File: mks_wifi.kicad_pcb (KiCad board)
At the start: 2 copper layers, 22.4 x 21.6 mm, 4 parts, among them J1 Conn_01x08, J2 Conn_01x08, U1 ESP-12F

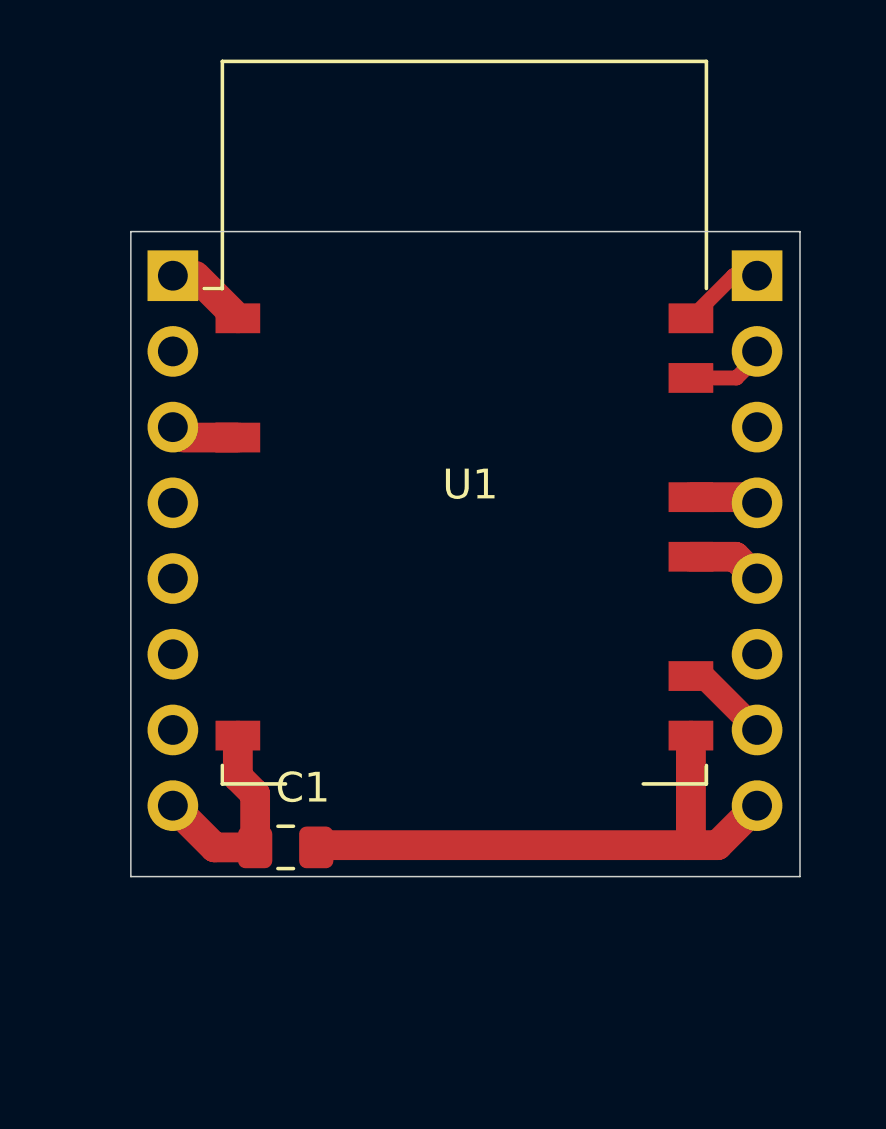
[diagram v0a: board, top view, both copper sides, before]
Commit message: v1, проверенный вариант
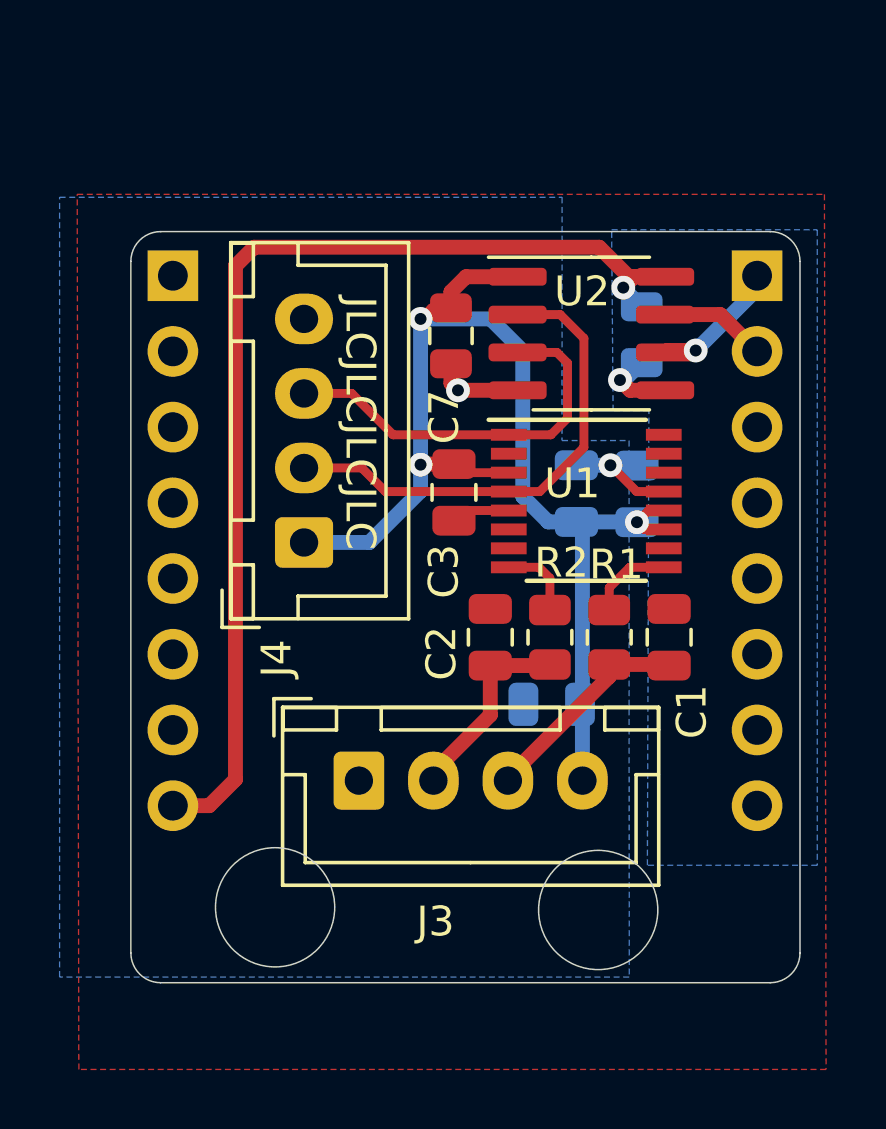
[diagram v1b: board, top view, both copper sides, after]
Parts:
- added C2: 47pF, Capacitor_SMD:C_0805_2012Metric, F.Cu at (174.6, 62.1)
- added C3: 0.1uF, Capacitor_SMD:C_0805_2012Metric, F.Cu at (173.4, 57.2)
- added C4: 4.7uF, Capacitor_SMD:C_0805_2012Metric, B.Cu at (177.5, 57.3)
- added C5: 0.1uF, Capacitor_SMD:C_0805_2012Metric, B.Cu at (179.5, 57.3)
- added C6: 0.01uF, Capacitor_SMD:C_0805_2012Metric, B.Cu at (176.7, 64.3)
- added C7: 1uF, Capacitor_SMD:C_0805_2012Metric, F.Cu at (173.3, 52.0)
- added C8: 1uF, Capacitor_SMD:C_0805_2012Metric, B.Cu at (179.7, 51.9)
- added J3: USB, Connector_JST:JST_XH_B4B-XH-A_1x04_P2.50mm_Vertical, F.Cu at (170.2, 66.9)
- added J4: UART, Connector_JST:JST_XH_B4B-XH-A_1x04_P2.50mm_Vertical, F.Cu at (168.4, 58.9)
- added R1: 27, Resistor_SMD:R_0805_2012Metric, F.Cu at (178.6, 62.1)
- added R2: 27, Resistor_SMD:R_0805_2012Metric, F.Cu at (176.6, 62.1)
- added U2: ISO7721, Package_SO:SOIC-8_3.9x4.9mm_P1.27mm, F.Cu at (178.0, 51.9)
- C1: value C_Small -> 47pF; footprint Capacitor_SMD:C_0805_2012Metric_Pad1.15x1.40mm_HandSolder -> Capacitor_SMD:C_0805_2012Metric
- U1: value ESP-12F -> FT230XS; footprint mks_wifi:ESP-12E_MKS -> Package_SO:SSOP-16_3.9x4.9mm_P0.635mm
- moved C1 14.7 mm to (180.6, 62.1), turned to 90 degrees
- moved U1 4.86 mm to (177.8, 57.5)
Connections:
- C1 pad 1: 3v3 -> USB_DM
- J1 pad 1: RST -> (no net)
- J1 pad 3: EN -> (no net)
- J1 pad 8: 3v3 -> 3V3
- J2 pad 4: IO2 -> (no net)
- J2 pad 5: IO1 -> (no net)
- J2 pad 7: 16 -> (no net)
- J2 pad 8: GND -> GND2
- U1 pad 1: RST -> Net-(J4-Pad3)
- U1 pad 15: GND -> (no net)
- U1 pad 16: 16 -> (no net)
- U1 pad 3: EN -> VDD_USB
- U1 pad 8: 3v3 -> Net-(R2-Pad1)
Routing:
- net VDD_USB: track 0.00 -> 41.5 mm, vias 0 -> 3
- net 3V3: track 0.00 -> 36.2 mm, vias 0 -> 1
- net Net-(J4-Pad2): track 0.00 -> 16.5 mm
- net Net-(J4-Pad3): track 0.00 -> 13.3 mm
- net GND: track 19.1 -> 9.16 mm, vias 0 -> 2
- net USB_DM: track 0.00 -> 7.33 mm
- net 3v3: track 7.26 -> 0.00 mm
- net USB_DP: track 0.00 -> 6.67 mm
- net 16: track 2.97 -> 0.00 mm
- net Net-(R1-Pad1): track 0.00 -> 2.86 mm
- net RST: track 2.77 -> 0.00 mm
- net GND2: track 0.00 -> 2.63 mm, vias 0 -> 1
- net Net-(R2-Pad1): track 0.00 -> 2.60 mm
- net IO1: track 2.52 -> 0.00 mm
- net EN: track 2.32 -> 0.00 mm
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- added copper zone on B.Cu, net GND
- added copper zone on F.Cu, net GND
- added copper zone on B.Cu, net GND2
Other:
- board size 22.4 x 21.6 mm -> 22.5 x 25.2 mm
- net class Default: clearance 0.3 -> 0.25
- rule trace_clearance: 0.3 -> 0.25
- board text added: "DM"
- board text added: "DP"
- board text added: "GND"
- board text added: "GND2"
- board text added: "JLCJLCJLCJLC"
- board text added: "RX"
- board text added: "TX"
- board text added: "VDD"
